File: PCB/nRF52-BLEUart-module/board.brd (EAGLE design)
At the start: 40 x 18 mm, 44 parts, among them J1 USB-A_PTH_MALE, U1 CH340E, U2 NRF52832, Y1 32MHz_2016, Y2 32.768kHz

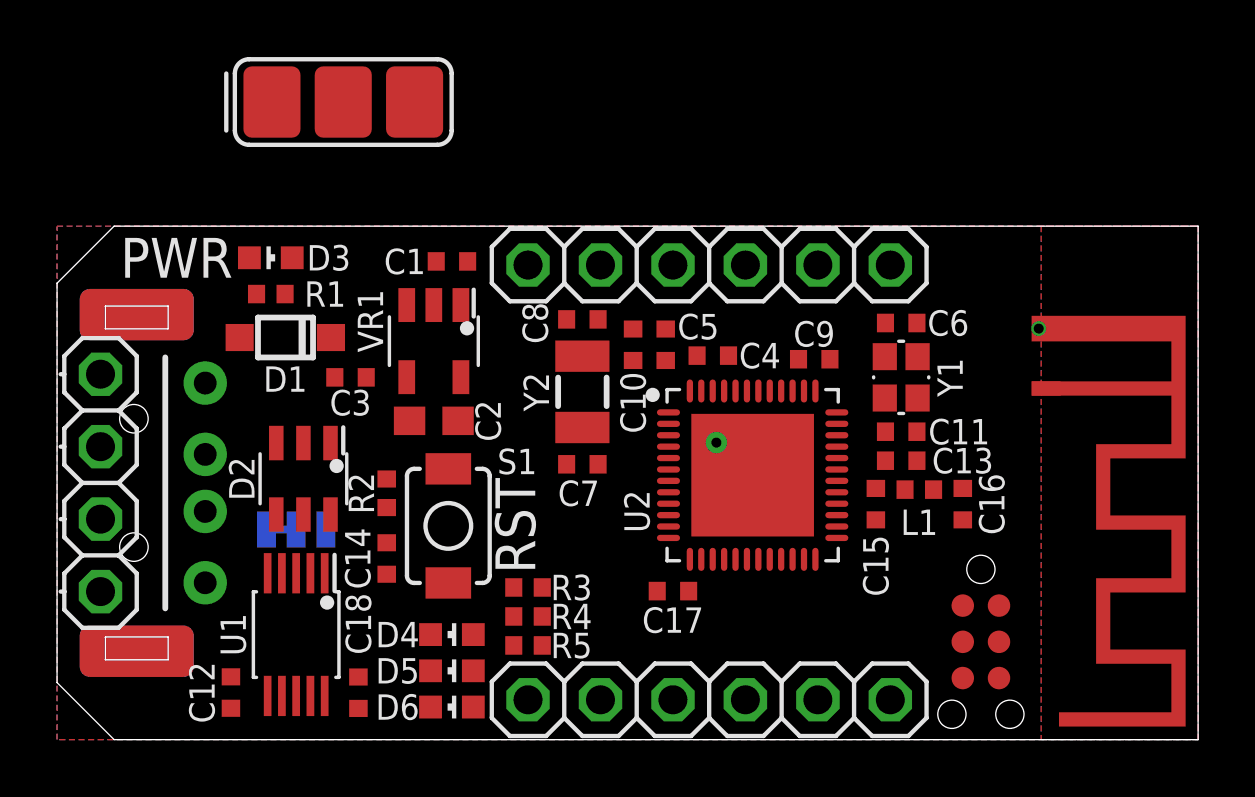
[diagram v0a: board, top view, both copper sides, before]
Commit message: artwork partially done, layout update
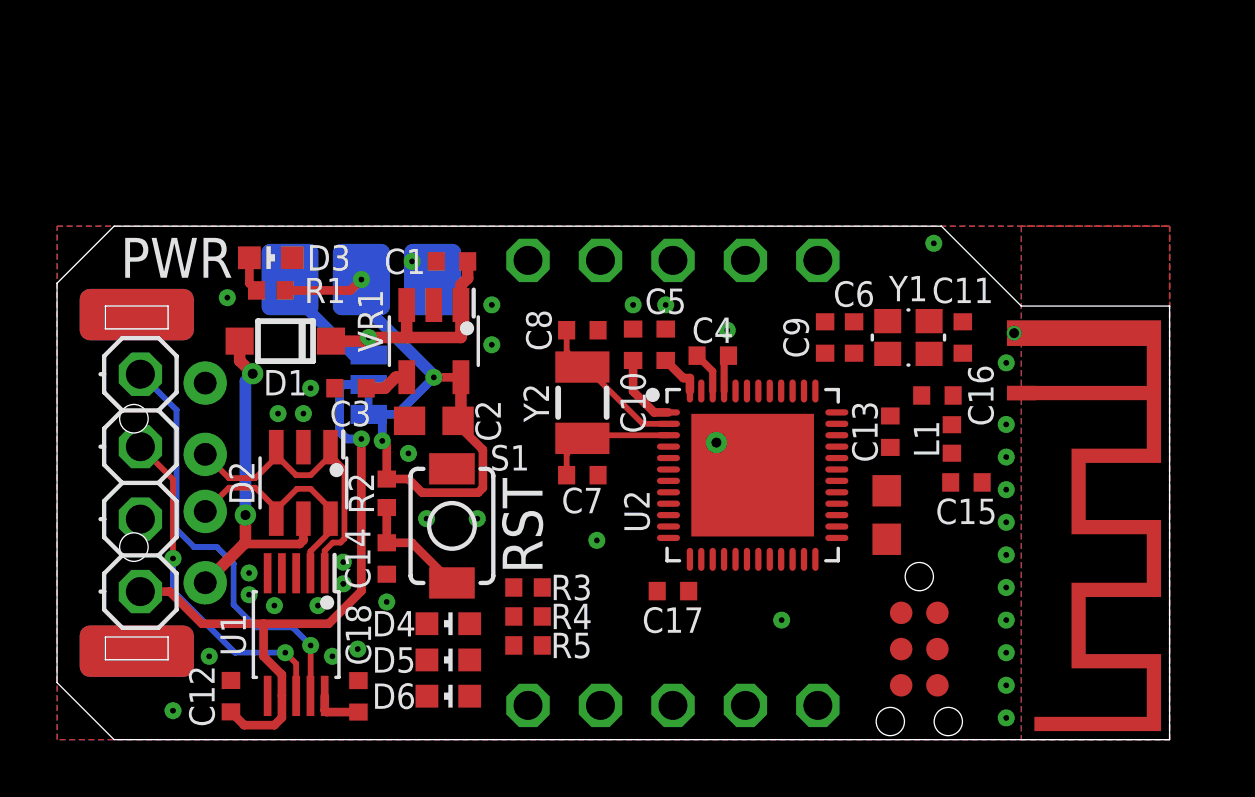
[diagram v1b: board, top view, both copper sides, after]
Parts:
- added C19: TP, angrypig7-RCL:C0603
- JP1: value V G Rx Tx -> V G Tx Rx
- JP3, JP4: device angrypig7-Connectors-PinHeads:1X06 -> angrypig7-Connectors-PinHeads:1X05-NOSILK
- moved TP1 6.26 mm to (10.7, 16.1), flipped to the bottom
- moved JP2 5.68 mm to (10.9, 12.4), turned to 270 degrees
- moved C11 3.95 mm to (31.8, 14.1), turned to 270 degrees
- moved C16 3.91 mm to (30.9, 12.1), turned to 180 degrees
- moved C15 3.27 mm to (31.9, 9.02), turned to 0 degrees
- moved TC1 2.17 mm to (30.2, 3.17)
- moved L1 2.11 mm to (31.4, 10.5), turned to 90 degrees
- moved C6 1.73 mm to (27.9, 14.1), turned to 90 degrees
- moved Y1 1.42 mm to (29.8, 14.1), turned to 180 degrees
- moved JP1 1.40 mm to (2.92, 9.00)
- moved JP4 1.29 mm to (21.6, 1.20)
- moved JP3 1.28 mm to (21.6, 16.8)
- moved C13 1.09 mm to (29.2, 10.8), turned to 90 degrees
- moved U$1 0.88 mm to (33.3, 14.7)
- moved C9 0.85 mm to (26.9, 14.1), turned to 90 degrees
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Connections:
- net N$2 renamed USB_IN
- removed net N$15: C12.1, JP2.2, U1.7
- new net VCCIO: C12.1, JP1.1, JP2.2, U1.7
- net 3V3: no longer JP1.1
- net GND: now also C19.2
- net RF-1: now also C19.1
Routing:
- net VCCIO: track 0.00 -> 23.1 mm, vias 0 -> 1
- net 3V3: track 0.00 -> 22.9 mm, vias 0 -> 3
- net UART_RX: track 0.00 -> 15.5 mm, vias 0 -> 1
- net 5V: track 0.00 -> 13.2 mm, vias 0 -> 1
- net USB_IN: track 0.00 -> 12.2 mm, vias 0 -> 2
- net UART_TX: track 0.00 -> 12.0 mm, vias 0 -> 2
- net USB_P: track 0.00 -> 11.3 mm
- net USB_N: track 0.00 -> 8.85 mm
- net N$1: track 0.00 -> 5.36 mm
- net N$4: track 0.00 -> 4.58 mm
- net NRST: track 0.00 -> 4.10 mm
- net N$5: track 0.00 -> 2.63 mm
- net N$16: track 0.00 -> 1.71 mm
- net N$3: track 0.00 -> 1.58 mm
- net N$7: track 0.00 -> 1.47 mm
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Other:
- board size 40 x 18 mm -> 39 x 18 mm
